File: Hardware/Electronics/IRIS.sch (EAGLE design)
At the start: 3 parts, among them X1 MINI-USB-32005-201

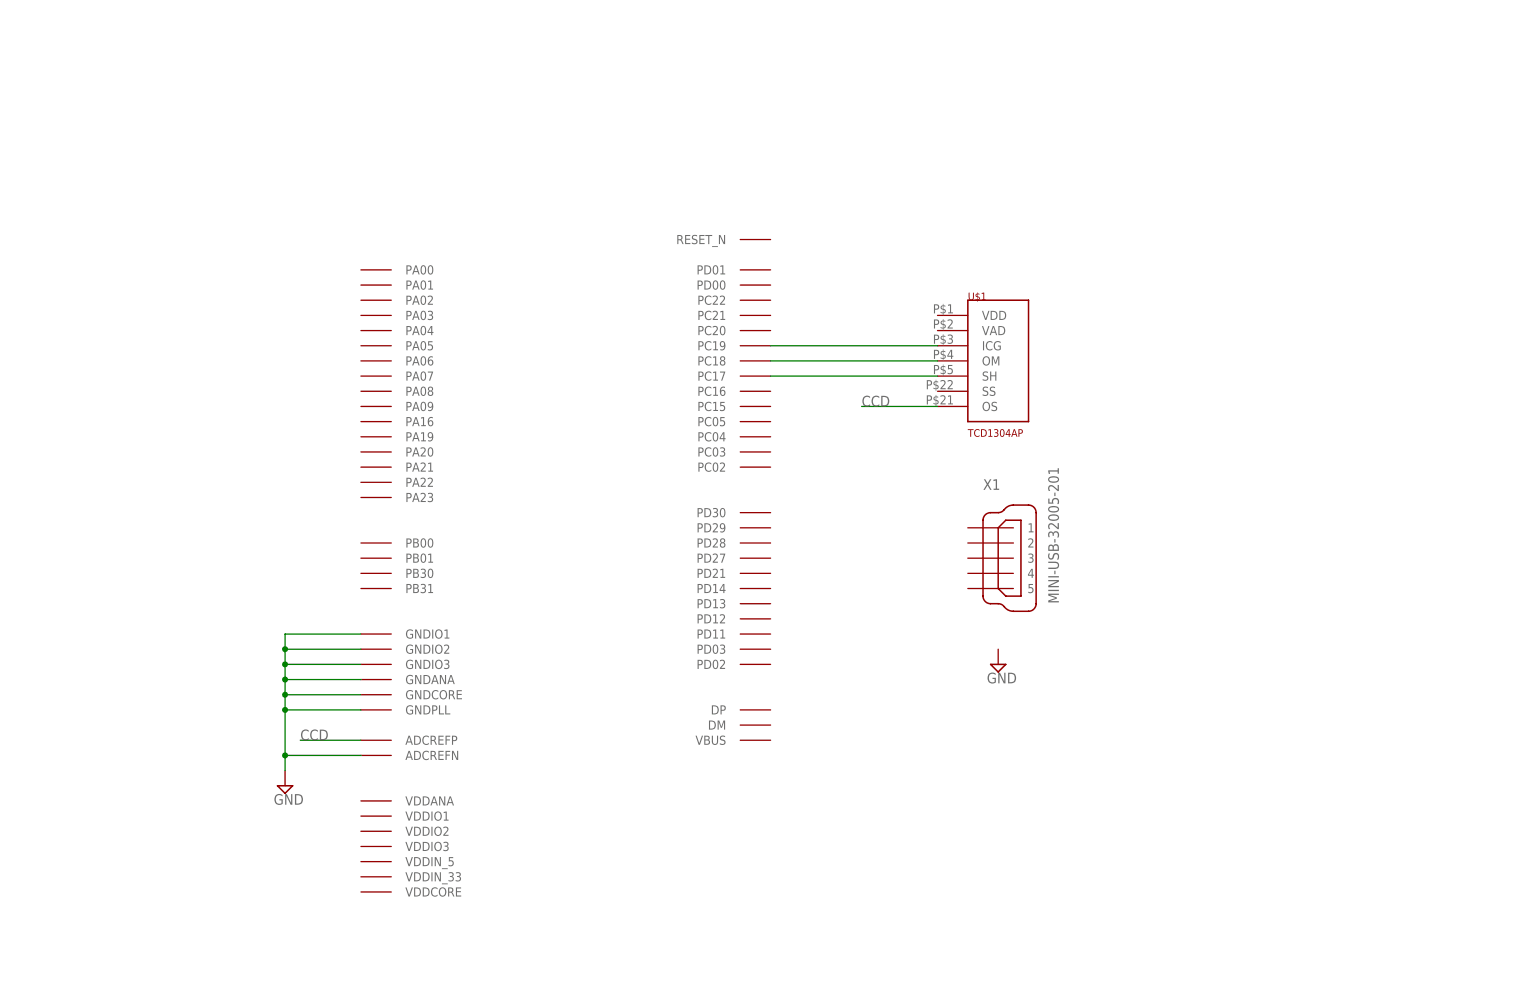
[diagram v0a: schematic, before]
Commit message: Schematic modifications…
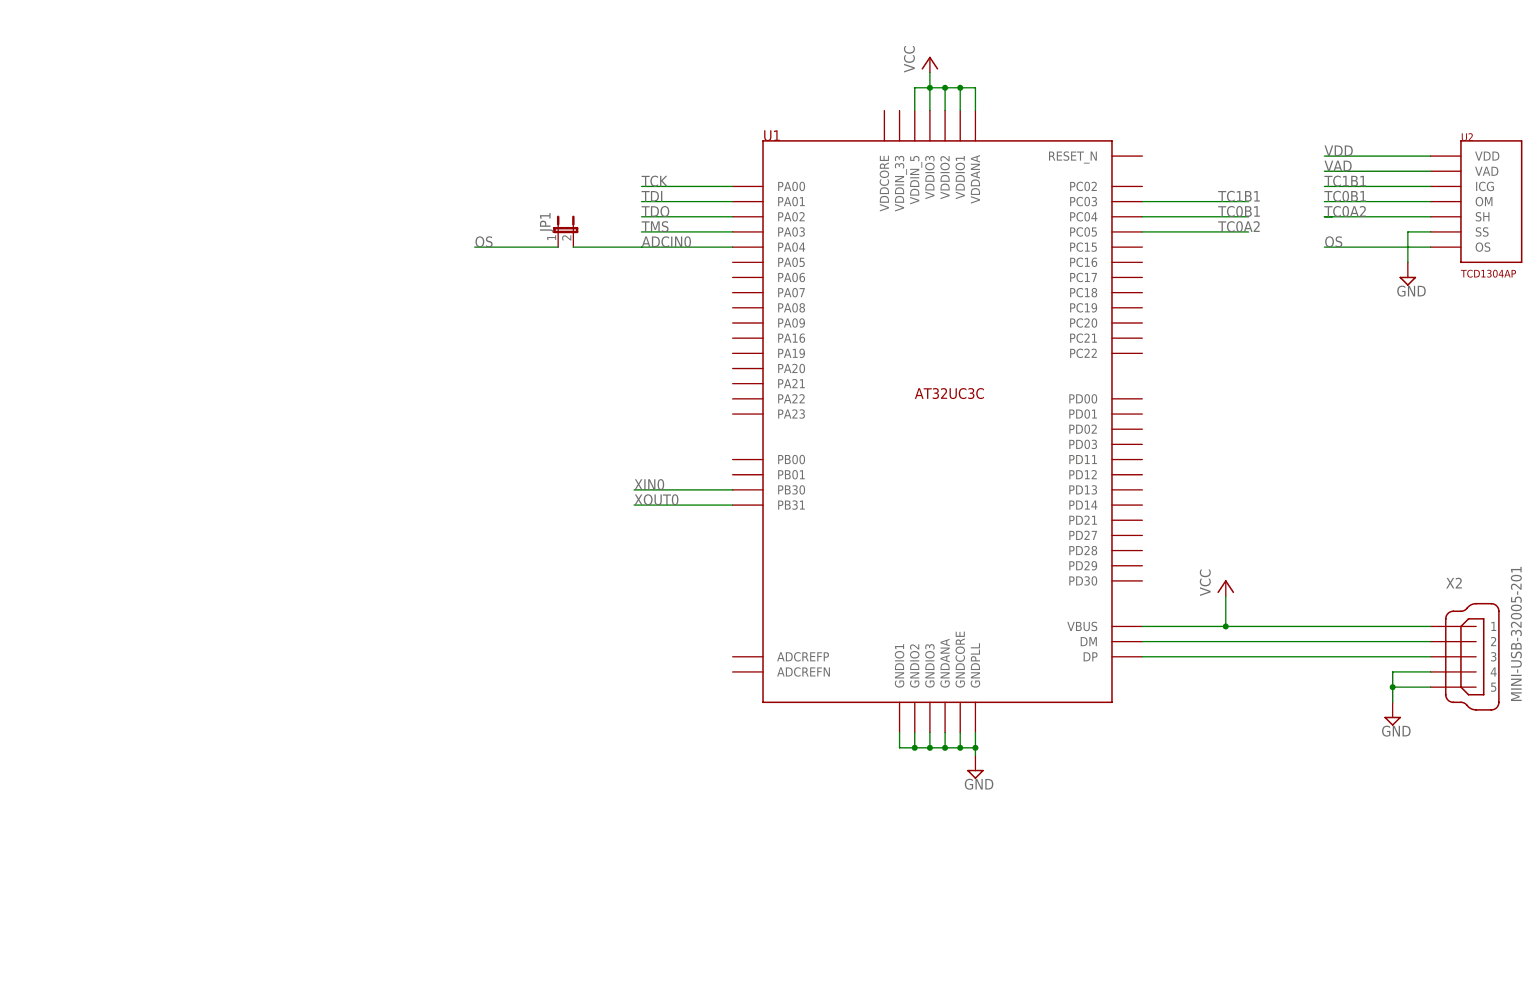
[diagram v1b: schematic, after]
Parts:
- removed U$1: TCD1304AP, SPectrolib:TCD1304AP
- removed U$2: AT32UC3C, SPectrolib:AT32UC3C
- removed X1: MINI-USB-32005-201, con-cypressindustries:MINI-USB-32005-201
- added JP1: (no value), jumper:JP1E
- added U1: AT32UC3C, IRIS:AT32UC3C
- added U2: TCD1304AP, IRIS:TCD1304AP
- added X2: MINI-USB-32005-201, con-cypressindustries:MINI-USB-32005-201
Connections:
- removed net CCD: U$1.OS, U$2.ADCREFP
- removed net N$3: U$1.SH, U$2.PC17
- new net ADCIN0: JP1.2, U1.PA04
- new net OS: JP1.1, U2.OS
- new net TC0A2: U1.PC05, U2.SH
- new net TC0B1: U1.PC04, U2.OM
- new net TC1B1: U1.PC03, U2.ICG
- new net TCK: U1.PA00
- new net TDI: U1.PA01
- new net TDO: U1.PA02
- new net TMS: U1.PA03
- new net VAD: U2.VAD
- new net VCC: U1.VBUS, U1.VDDANA, U1.VDDIN_5, U1.VDDIO1, U1.VDDIO2, U1.VDDIO3, X2.1
- new net VDD: U2.VDD
- new net XIN0: U1.PB30
- new net XOUT0: U1.PB31
- net GND: now also U1.GNDANA, U1.GNDCORE, U1.GNDIO1, U1.GNDIO2, U1.GNDIO3, U1.GNDPLL, U2.SS, X2.4, X2.5; no longer U$2.ADCREFN, U$2.GNDANA, U$2.GNDCORE, U$2.GNDIO1, U$2.GNDIO2, U$2.GNDIO3, U$2.GNDPLL
- net N$1: now also U1.DM, X2.2; no longer U$1.ICG, U$2.PC19
- net N$2: now also U1.DP, X2.3; no longer U$1.OM, U$2.PC18

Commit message: Board routed.
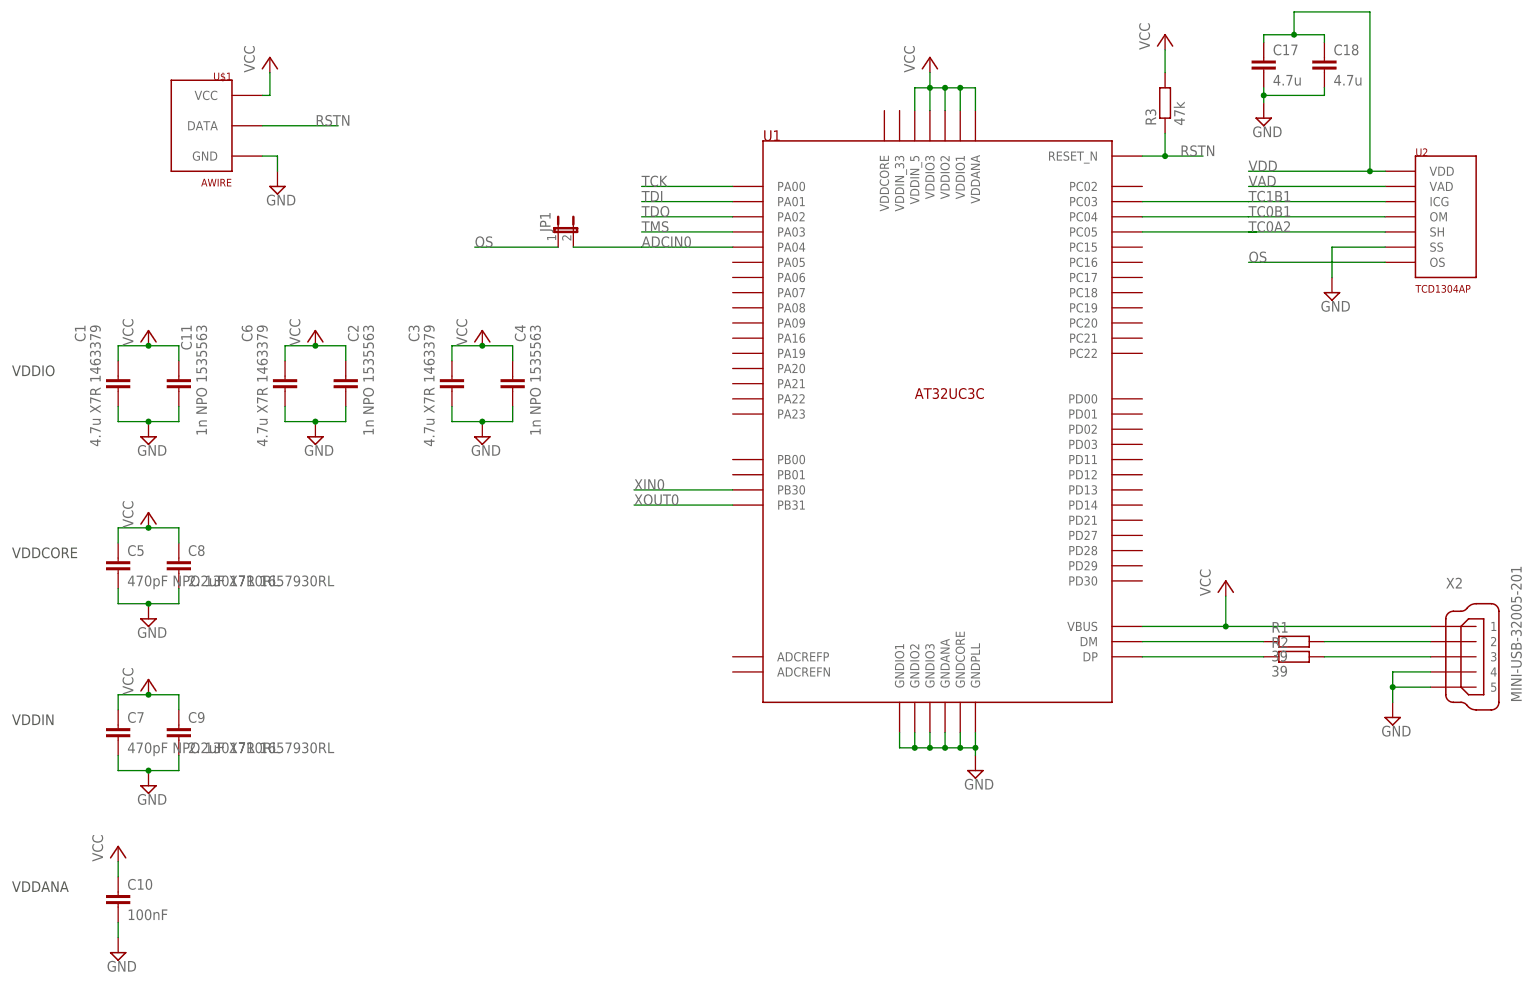
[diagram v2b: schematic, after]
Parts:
- added C1, C3, C6: 4.7u X7R 1463379, rcl:C-EUC0603
- added C10: 100nF, rcl:C-EUC0603
- added C11, C2, C4: 1n NPO 1535563, rcl:C-EUC0402
- added C17, C18: 4.7u, resistor:C-EUC0805
- added C5, C7: 470pF NPO 1301710RL, rcl:C-EUC0603
- added C8, C9: 2.2uF X7R 1657930RL, rcl:C-EUC0603
- added R1, R2: 39, rcl:R-EU_R0603
- added R3: 47k, rcl:R-EU_R0603
- added U$1: AWIRE, IRIS:AWIRE
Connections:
- new net N$3: R1.2, X2.2
- new net N$4: R2.2, X2.3
- new net RSTN: R3.1, U$1.DATA, U1.RESET_N
- net GND: now also C1.2, C10.2, C11.2, C17.2, C18.2, C2.2, C3.2, C4.2, C5.2, C6.2, C7.2, C8.2, C9.2, U$1.GND
- net N$1: now also R1.1; no longer X2.2
- net N$2: now also R2.1; no longer X2.3
- net VCC: now also C1.1, C10.1, C11.1, C2.1, C3.1, C4.1, C5.1, C6.1, C7.1, C8.1, C9.1, R3.2, U$1.VCC
- net VDD: now also C17.1, C18.1
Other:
- note added: "VDDANA"
- note added: "VDDCORE"
- note added: "VDDIN"
- note added: "VDDIO"
- moved on the sheet: U2
